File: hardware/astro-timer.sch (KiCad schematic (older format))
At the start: 23 parts, among them J1 Conn_01x02_Male, J2 AVR-ISP-6, J3 SJ1-2503A, SW1 SW_SPST, SW2 SW_Push, SW3 SW_Push, U1 ATmega328P-PU, U2 LTV-817M, U3 EN11-HSM1AF15, Y1 Crystal

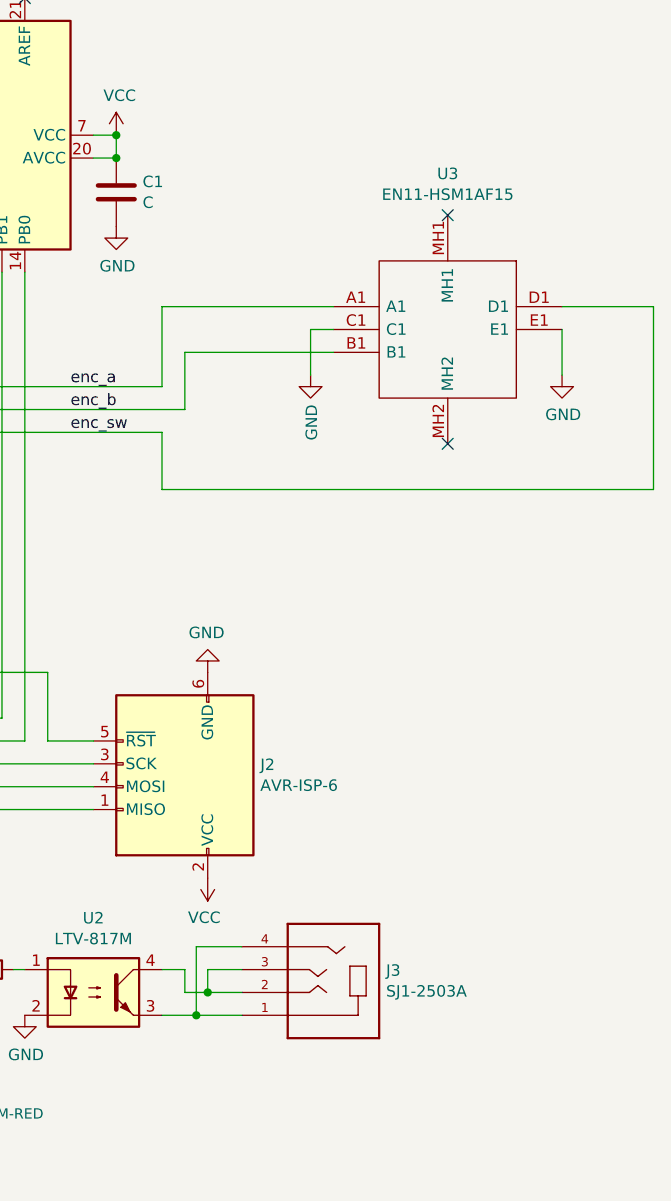
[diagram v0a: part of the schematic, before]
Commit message: moar pcb tweaks
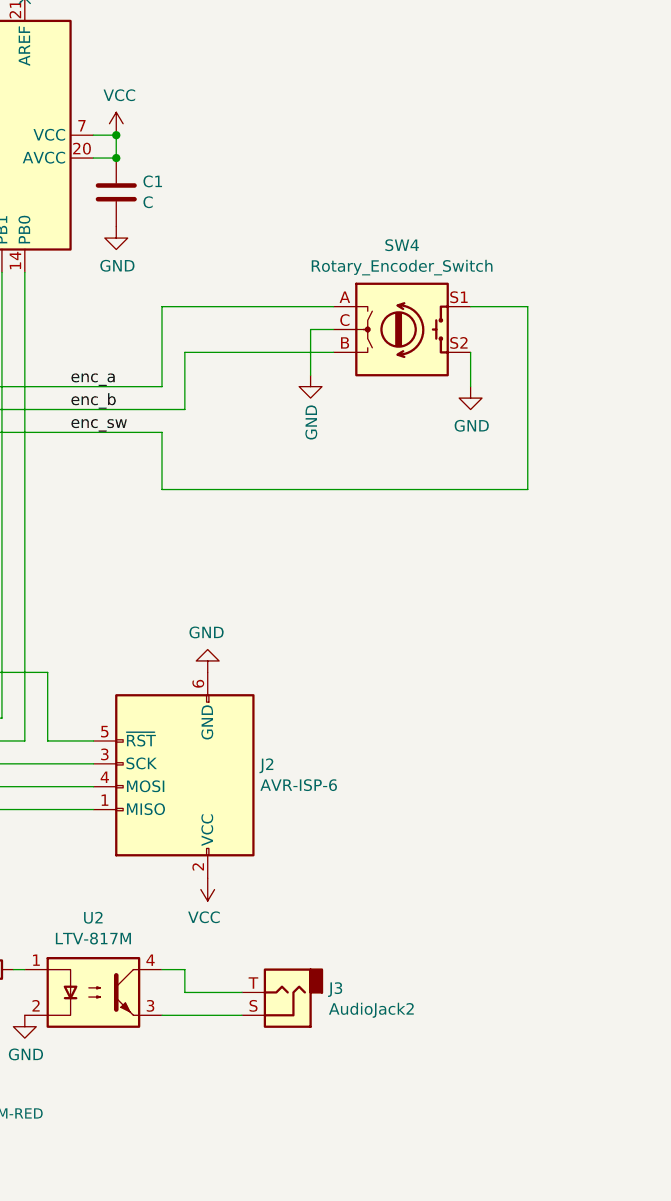
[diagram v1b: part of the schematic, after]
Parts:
- removed J3: SJ1-2503A, more_different_sj1:CUI_SJ1-2503A, symbol sj1-2503a:SJ1-2503A
- removed U3: EN11-HSM1AF15, en11:EN11HSM1AF15, symbol en11:EN11-HSM1AF15
- added J3: AudioJack2, more_different_sj1:CUI_SJ1-2503A, symbol Connector:AudioJack2
- added SW4: Rotary_Encoder_Switch, en11:EN11HSM1AF15, symbol Device:Rotary_Encoder_Switch
- SW1: footprint eg1218:EG1218 -> digikey:Switch_Slide_11.6x4mm_EG1218
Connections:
- net GND: now also SW4.C, SW4.S2
- net enc_a: now also SW4.A
- net enc_b: now also SW4.B
- net enc_sw: now also SW4.S1
- net at U2.3: now also J3.S
- net at U2.4: now also J3.T
- no-connect marks 3 -> 1
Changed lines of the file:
@@
 L power:GND #PWR012
 U 1 1 60408112
-P 9550 3000
-F 0 "#PWR012" H 9550 2750 50  0001 C CNN
-F 1 "GND" H 9555 2827 50  0000 C CNN
-F 2 "" H 9550 3000 50  0001 C CNN
-F 3 "" H 9550 3000 50  0001 C CNN
-	1    9550 3000
+P 9150 3050
+F 0 "#PWR012" H 9150 2800 50  0001 C CNN
+F 1 "GND" H 9155 2877 50  0000 C CNN
+F 2 "" H 9150 3050 50  0001 C CNN
+F 3 "" H 9150 3050 50  0001 C CNN
+	1    9150 3050
 	1    0    0    -1
 $EndComp
@@
 F 0 "SW1" H 3350 1535 50  0000 C CNN
 F 1 "SW_SPST" H 3350 1444 50  0000 C CNN
-F 2 "eg1218:EG1218" H 3350 1300 50  0001 C CNN
+F 2 "digikey:Switch_Slide_11.6x4mm_EG1218" H 3350 1300 50  0001 C CNN
 F 3 "~" H 3350 1300 50  0001 C CNN
 	1    3350 1300
@@
 Wire Wire Line
 	3550 1300 3650 1300
-$Comp
-L sj1-2503a:SJ1-2503A J3
-U 1 1 60401D7D
-P 8550 5600
-F 0 "J3" H 8320 5604 50  0000 R CNN
-F 1 "SJ1-2503A" H 8320 5695 50  0000 R CNN
-F 2 "more_different_sj1:CUI_SJ1-2503A" H 8550 5600 50  0001 L BNN
-F 3 "" H 8550 5600 50  0001 L BNN
-F 4 "B" H 8550 5600 50  0001 L BNN "REV"
-F 5 "Manufacturer Recommendation" H 8550 5600 50  0001 L BNN "STANDARD"
-F 6 "CUI INC" H 8550 5600 50  0001 L BNN "MANUFACTURER"
-	1    8550 5600
-	-1   0    0    1
-$EndComp
-$Comp
-L en11:EN11-HSM1AF15 U3
-U 1 1 6040D732
-P 9050 2300
-F 0 "U3" V 8869 2300 50  0000 C CNN
-F 1 "EN11-HSM1AF15" V 8960 2300 50  0000 C CNN
-F 2 "en11:EN11HSM1AF15" H 9900 2600 50  0001 L CNN
-F 3 "http://www.mouser.com/datasheet/2/414/Datasheet_RotaryEncoder_EN11Series-1154703.pdf" H 9900 2500 50  0001 L CNN
-F 4 "BI TECHNOLOGIES / TT ELECTRONICS - EN11-HSM1AF15 - INCREMENTAL ENCODER" H 9900 2400 50  0001 L CNN "Description"
-F 5 "22.1" H 9900 2300 50  0001 L CNN "Height"
-F 6 "BI Technologies" H 9900 2200 50  0001 L CNN "Manufacturer_Name"
-F 7 "EN11-HSM1AF15" H 9900 2100 50  0001 L CNN "Manufacturer_Part_Number"
-F 8 "858-EN11-HSM1AF15" H 9900 2000 50  0001 L CNN "Mouser Part Number"
-F 9 "https://www.mouser.co.uk/ProductDetail/BI-Technologies-TT-Electronics/EN11-HSM1AF15/?qs=u1MaZ2%2F4xgsleMatSs8Sqg%3D%3D" H 9900 1900 50  0001 L CNN "Mouser Price/Stock"
-F 10 "EN11-HSM1AF15" H 9900 1800 50  0001 L CNN "Arrow Part Number"
-F 11 "https://www.arrow.com/en/products/en11-hsm1af15/bi-technologies" H 9900 1700 50  0001 L CNN "Arrow Price/Stock"
-	1    9050 2300
-	0    1    1    0
-$EndComp
 Wire Wire Line
-	9550 2700 9950 2700
+	9150 2700 9400 2700
 Wire Wire Line
-	9950 2700 9950 3500
+	9400 2700 9400 3500
 Wire Wire Line
-	9950 3500 7800 3500
+	9400 3500 7800 3500
 Wire Wire Line
 	7800 3500 7800 3250
@@
 	8450 2800 8450 3000
 Wire Wire Line
-	9550 2800 9550 3000
-NoConn ~ 9050 3300
-NoConn ~ 9050 2300
-Wire Wire Line
-	7900 5700 8000 5700
-Wire Wire Line
-	7800 5800 7950 5800
-Wire Wire Line
-	8150 5500 7950 5500
-Wire Wire Line
-	7950 5500 7950 5800
-Connection ~ 7950 5800
-Wire Wire Line
-	7950 5800 8150 5800
-Wire Wire Line
-	8150 5600 8000 5600
-Wire Wire Line
-	8000 5600 8000 5700
-Connection ~ 8000 5700
-Wire Wire Line
-	8000 5700 8150 5700
+	9150 2900 9150 3050
 $Comp
 L Connector:Conn_01x02_Male J1
@@
 Wire Wire Line
 	5800 2700 5800 2550
+$Comp
+L Connector:AudioJack2 J3
+U 1 1 603FA50D
+P 8350 5700
+F 0 "J3" H 8170 5683 50  0000 R CNN
+F 1 "AudioJack2" H 8170 5774 50  0000 R CNN
+F 2 "more_different_sj1:CUI_SJ1-2503A" H 8350 5700 50  0001 C CNN
+F 3 "~" H 8350 5700 50  0001 C CNN
+	1    8350 5700
+	-1   0    0    1
+$EndComp
+Wire Wire Line
+	7800 5800 8150 5800
+Wire Wire Line
+	7900 5700 8150 5700
+$Comp
+L Device:Rotary_Encoder_Switch SW4
+U 1 1 6041992A
+P 8850 2800
+F 0 "SW4" H 8850 3167 50  0000 C CNN
+F 1 "Rotary_Encoder_Switch" H 8850 3076 50  0000 C CNN
+F 2 "en11:EN11HSM1AF15" H 8700 2960 50  0001 C CNN
+F 3 "~" H 8850 3060 50  0001 C CNN
+	1    8850 2800
+	1    0    0    -1
+$EndComp
 $EndSCHEMATC
